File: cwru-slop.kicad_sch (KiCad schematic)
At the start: 40 parts, among them J1 USB_C_Receptacle_USB2.0_16P, SW1 SW_SPDT, U1 TLV9001IDCK, U10 B3U-1000P, U2 AP63205WU, U3 TLV75533PDBV, U4 STM32L433CCTx, U5 TPS2116DRL, U6 FXLS8974CFR3, U7 ESDCAN24-2BLY, U8 MCP2562-E-SN, U9 24lc32at-i/ot, Y1 XRCGB24M000F3M00R0

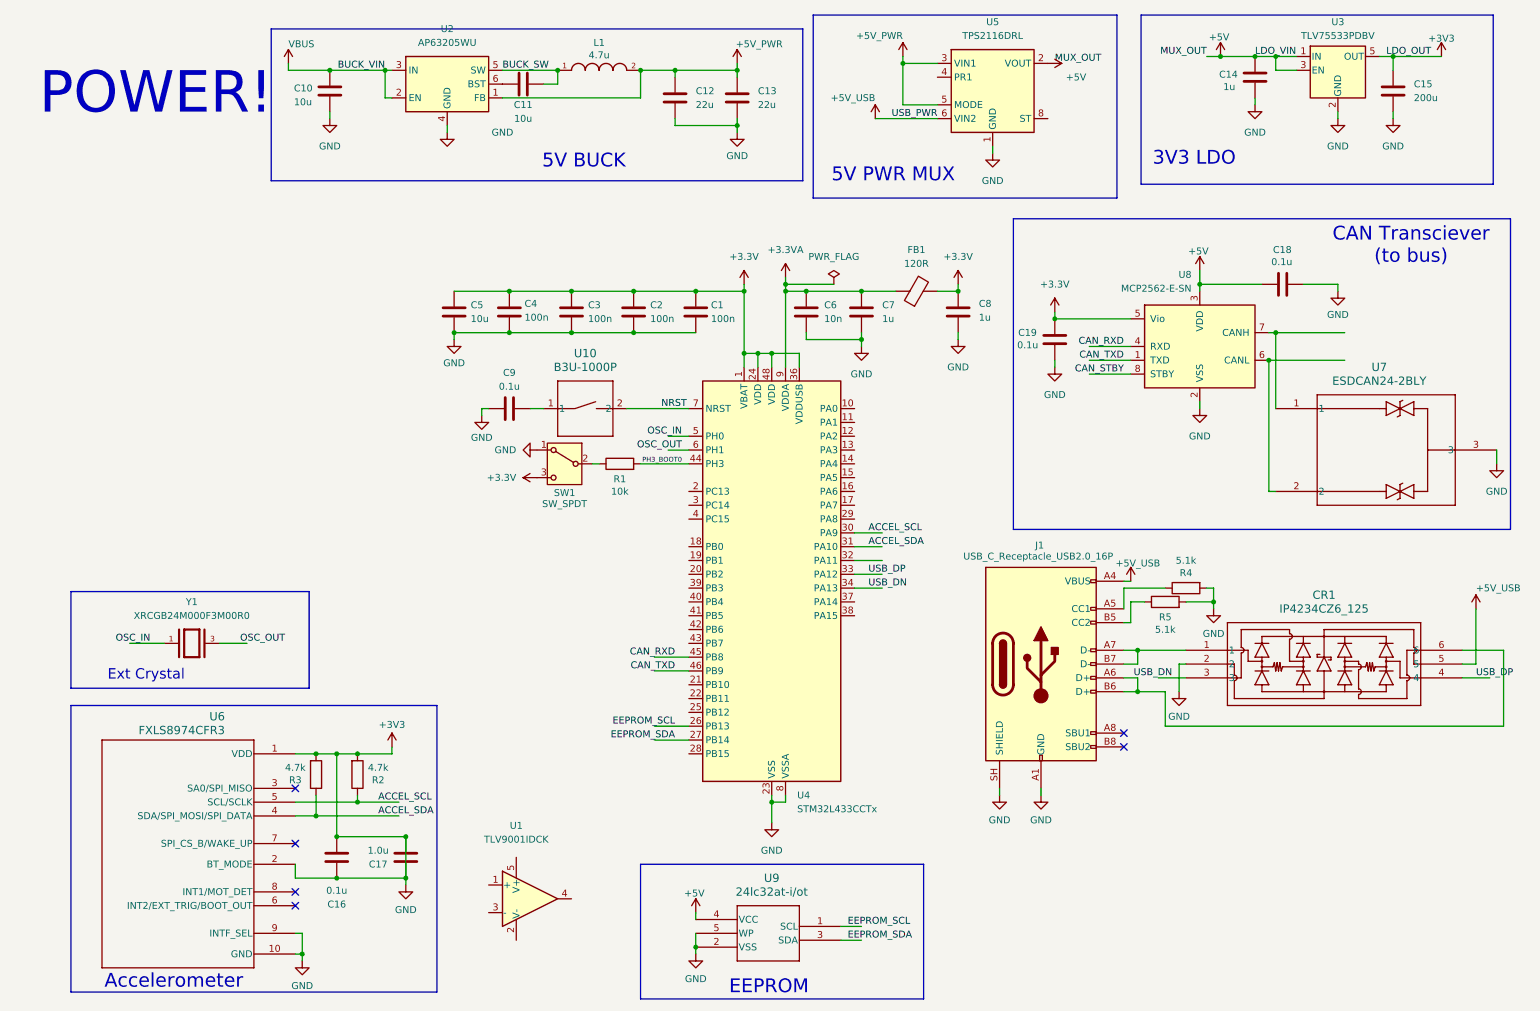
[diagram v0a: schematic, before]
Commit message: rotate usb diode, org
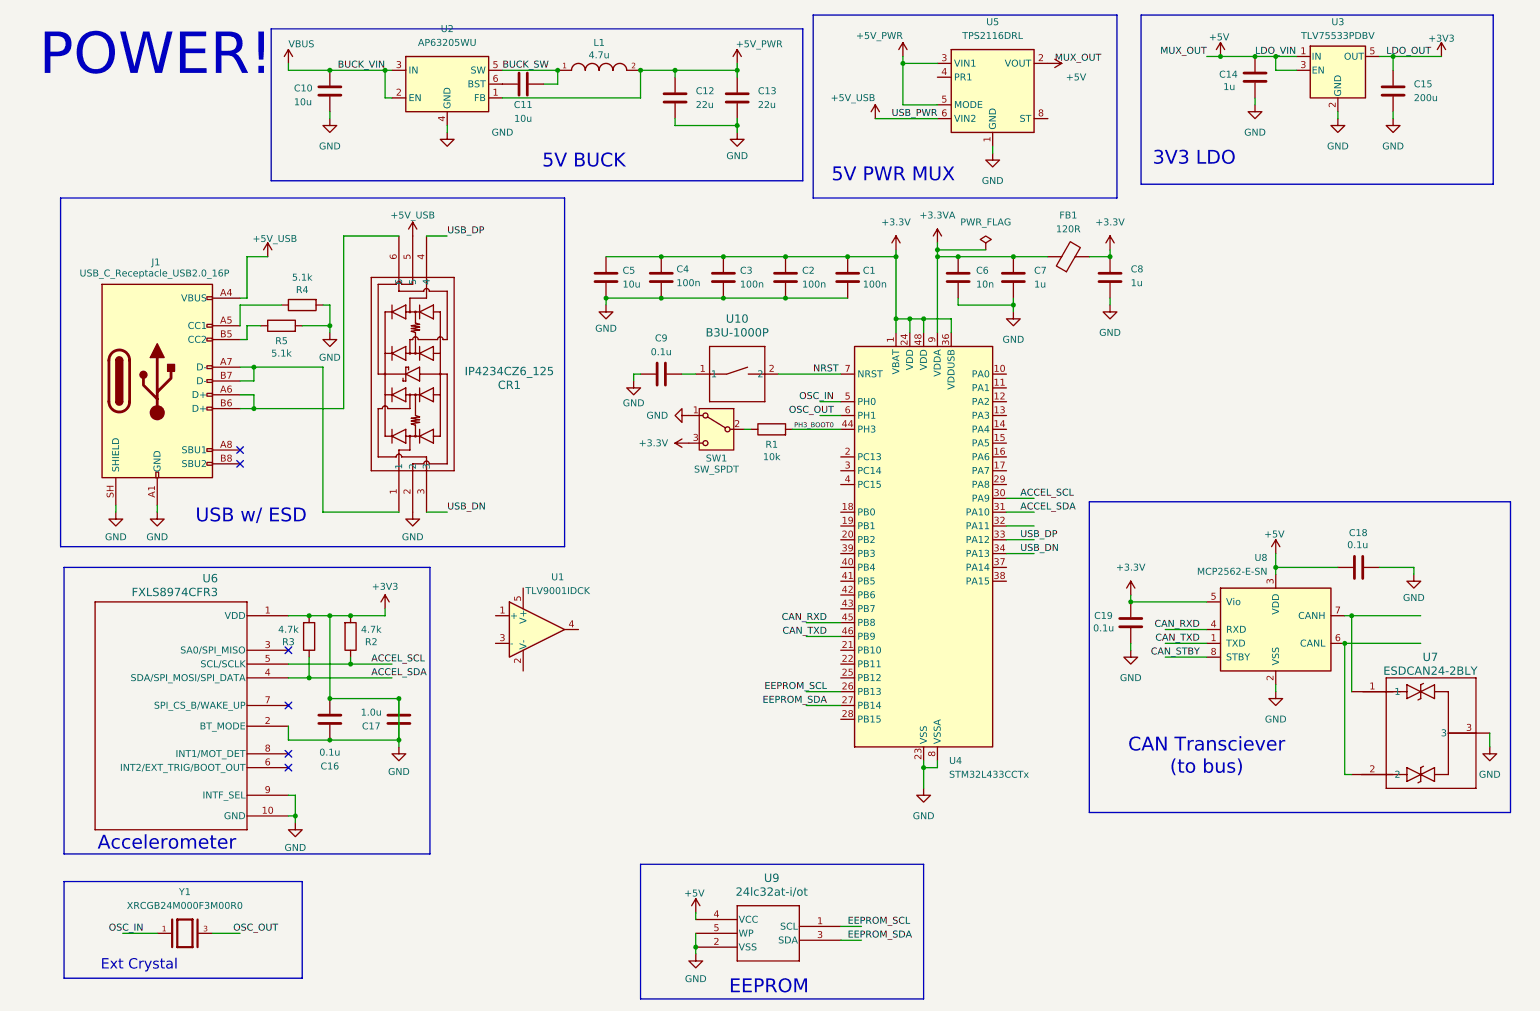
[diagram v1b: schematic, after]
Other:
- note added: "USB w/ ESD"
- moved on the sheet: C1, C16, C17, C18, C19, C2, C3, C4, C5, C6, C7, C8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
